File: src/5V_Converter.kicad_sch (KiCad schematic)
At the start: 16 parts, among them U3 TPS566238RQFR

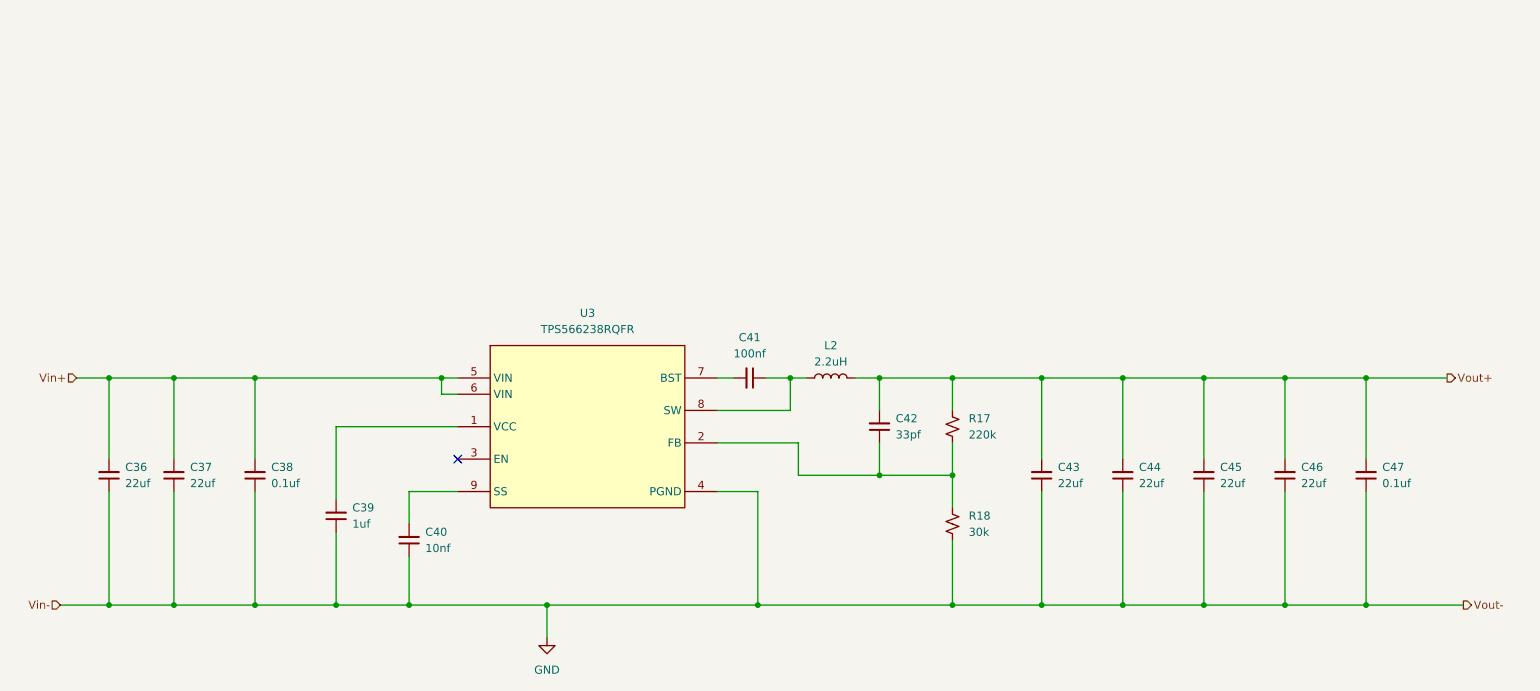
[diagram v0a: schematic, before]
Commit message: GG
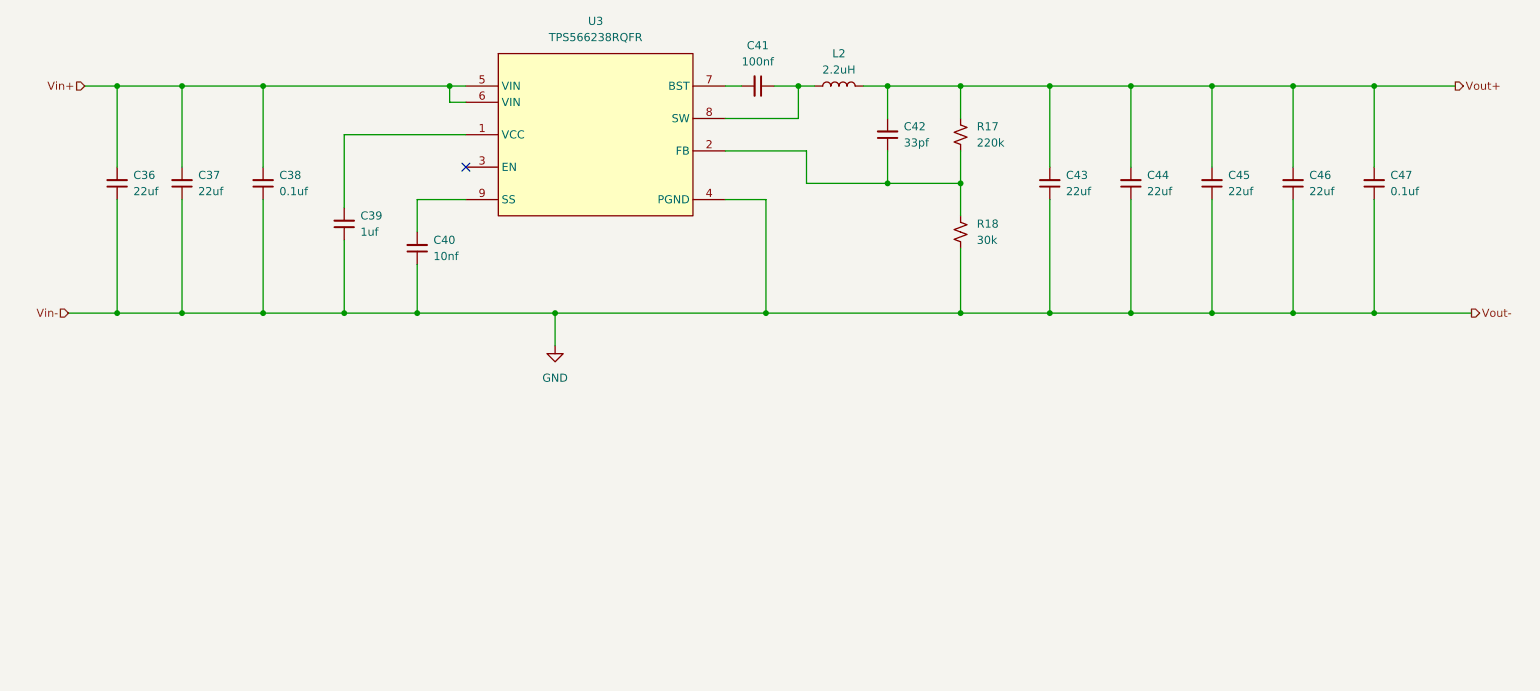
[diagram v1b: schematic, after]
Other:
- moved on the sheet: C36, C37, C38, C39, C40, C41, C42, C43, C44, C45, C46, C47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

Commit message: Completed half of the PCB layout
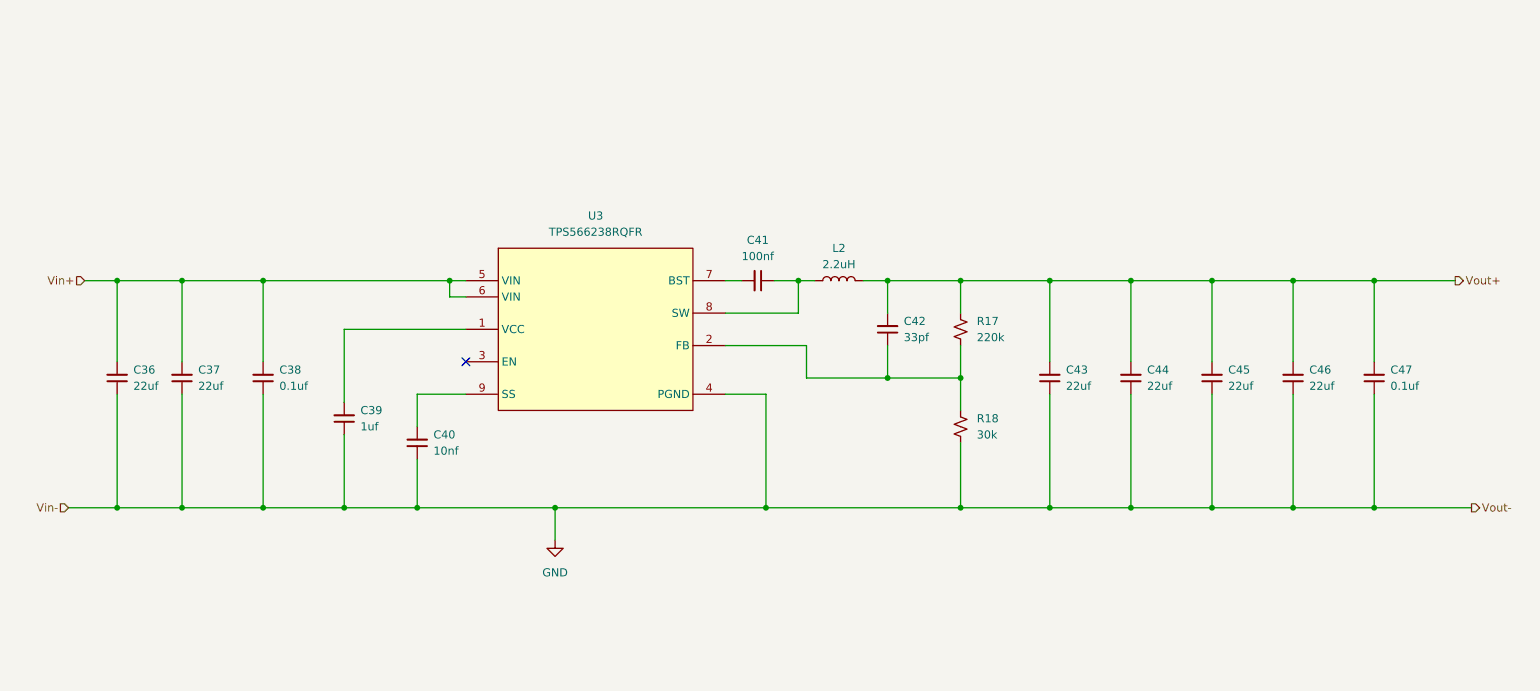
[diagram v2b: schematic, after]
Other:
- moved on the sheet: C36, C37, C38, C39, C40, C41, C42, C43, C44, C45, C46, C47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

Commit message: Upated parts and BOM
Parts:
- C36, C37, C43, C44, C45, C46: LCSC Part (none) -> C5677683; MPN (none) -> MSAST21GBB5226MTNC12; Manufacturer (none) -> Taiyo Yuden
- C38, C47: LCSC Part (none) -> C108079; MPN (none) -> CC0603KRX7R7BB104; Manufacturer (none) -> YAGEO
- C39: LCSC Part (none) -> C2180996; MPN (none) -> C0603C105Z8VACTU; Manufacturer (none) -> KEMET
- C40: LCSC Part (none) -> C85735; MPN (none) -> GRM155R71C103KA01D; Manufacturer (none) -> Murata Electronics
- C41: LCSC Part (none) -> C71629; MPN (none) -> GRM155R71C104KA88D; Manufacturer (none) -> Murata Electronics
- C42: LCSC Part (none) -> C513616; MPN (none) -> CC0201JRNPO8BN330; Manufacturer (none) -> YAGEO
- L2: LCSC Part (none) -> C5337632; MPN (none) -> DR125-2R2-R; Manufacturer (none) -> EATON
- R17: LCSC Part (none) -> C123420; MPN (none) -> RC0603FR-07220KL; Manufacturer (none) -> YAGEO
- R18: LCSC Part (none) -> C100001; MPN (none) -> RC0603FR-0730KL; Manufacturer (none) -> YAGEO
- U3: LCSC Part (none) -> C5219353; MPN (none) -> TPS566238RQFR; Manufacturer (none) -> Texas Instruments
